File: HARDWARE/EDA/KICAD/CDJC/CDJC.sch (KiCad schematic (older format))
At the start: 68 parts

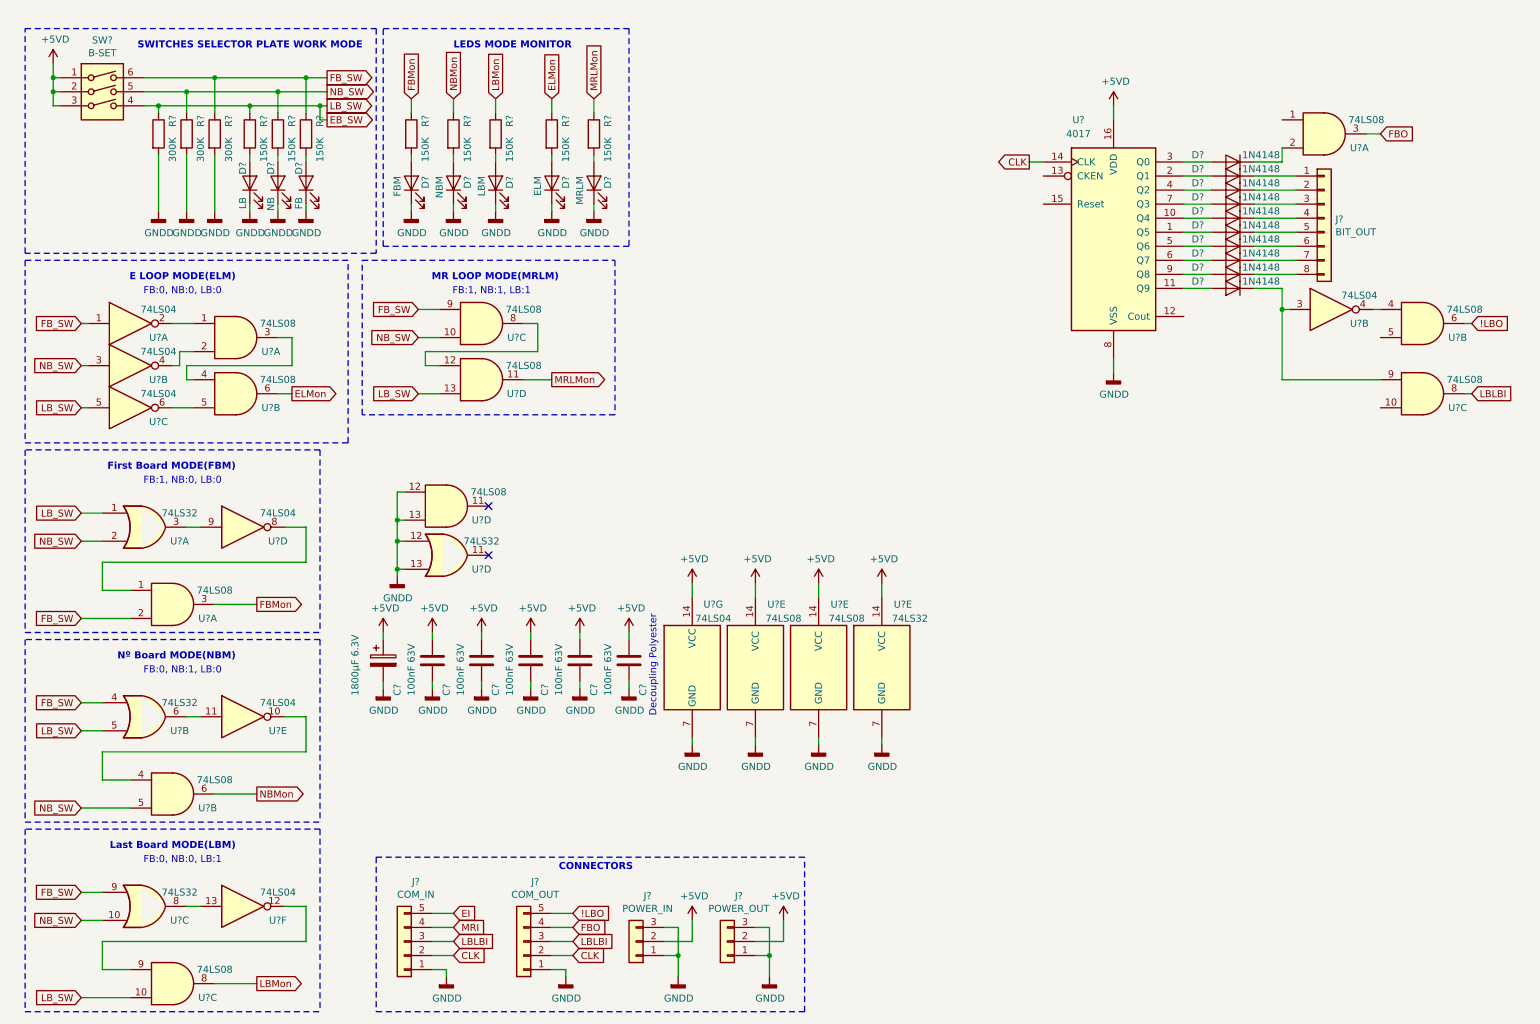
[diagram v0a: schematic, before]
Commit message: finished project
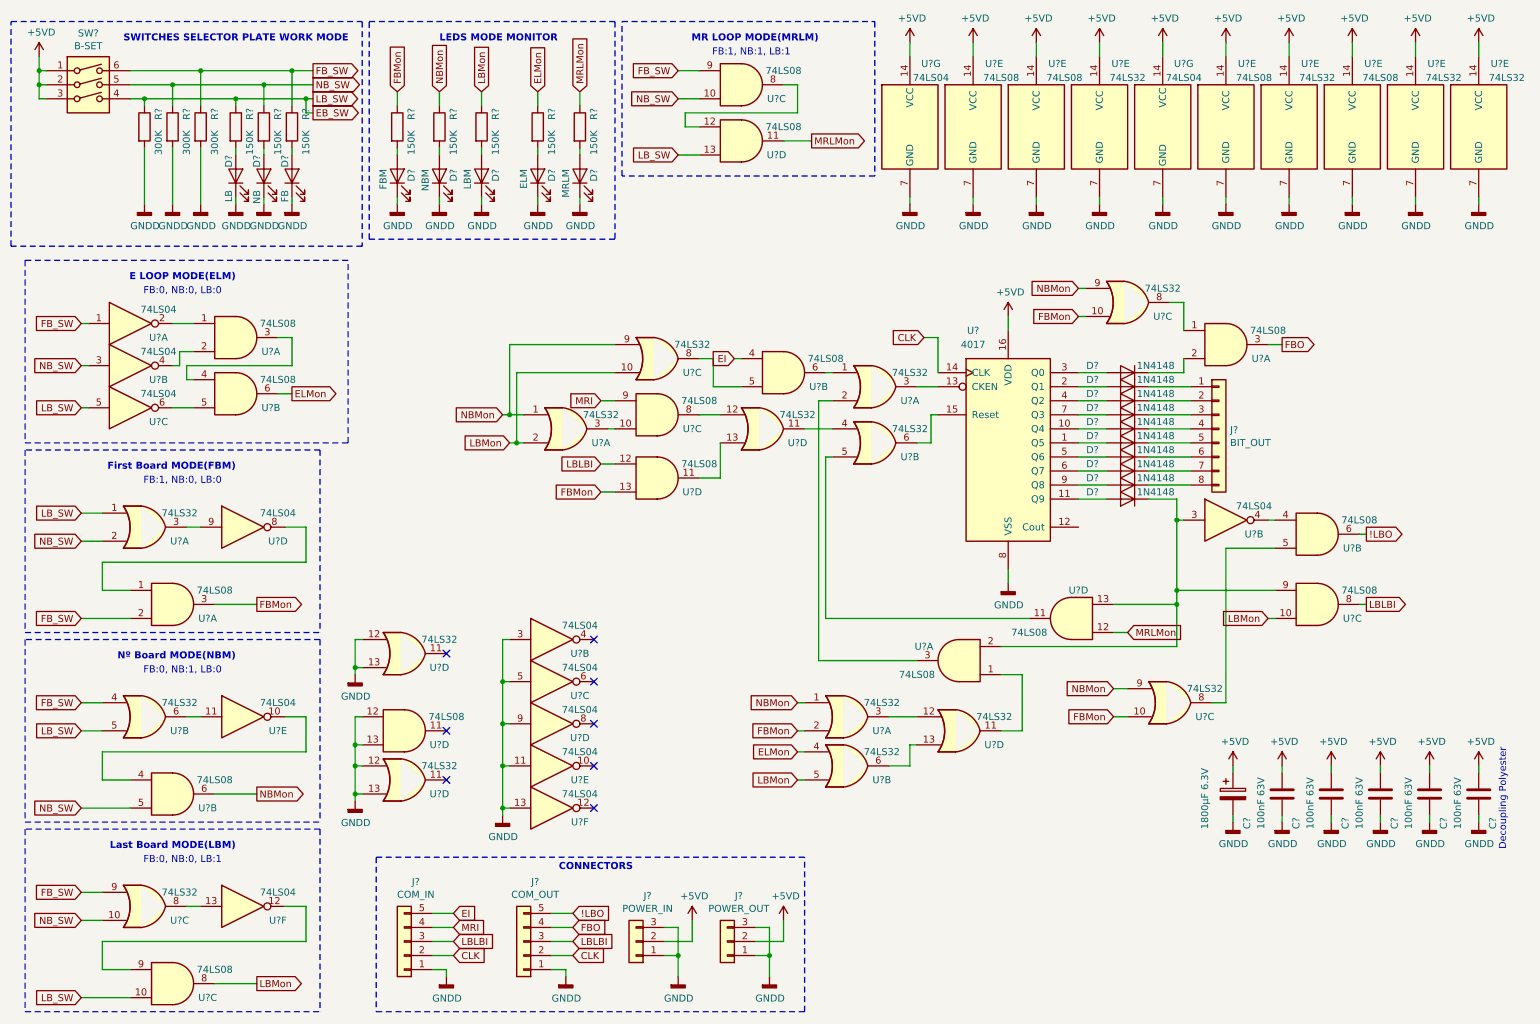
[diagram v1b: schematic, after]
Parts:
- added U? (x14): 74LS32, symbol 74xx:74LS32
- added U? (x7): 74LS08, symbol 74xx:74LS08
- added U? (x6): 74LS04, symbol 74xx:74LS04
- J?: footprint Connector_PinHeader_2.00mm:PinHeader_1x03_P2.00mm_Horizontal -> Connector_PinSocket_2.00mm:PinSocket_1x03_P2.00mm_Horizontal
- J?: footprint Connector_PinHeader_2.00mm:PinHeader_1x05_P2.00mm_Horizontal -> Connector_PinSocket_2.00mm:PinSocket_1x05_P2.00mm_Horizontal
- J?: footprint Connector_PinHeader_2.00mm:PinHeader_1x08_P2.00mm_Horizontal -> Connector_PinSocket_2.00mm:PinSocket_1x08_P2.00mm_Horizontal
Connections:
- net +5VD: now also U?.14 (VCC), U?.14 (VCC), U?.14 (VCC), U?.14 (VCC), U?.14 (VCC), U?.14 (VCC)
- net EI: now also U?.4
- net ELMon: now also U?.4
- net FBMon: now also U?.10, U?.10, U?.13, U?.2
- net GNDD: now also U?.11, U?.12, U?.13, U?.13, U?.3, U?.5, U?.7 (GND), U?.7 (GND), U?.7 (GND), U?.7 (GND), U?.7 (GND), U?.7 (GND), U?.9
- net LBLBI: now also U?.12
- net LBMon: now also U?.10, U?.10, U?.2, U?.5
- net MRI: now also U?.9
- net MRLMon: now also U?.12
- net NBMon: now also U?.1, U?.1, U?.9, U?.9, U?.9
- net at U?.13 (CKEN): now also U?.3
- net at U?.15 (Reset): now also U?.6
- net at D?.1 (K), U?.3, U?.9: now also U?.13, U?.2
- net at U?.5: now also U?.8
- net at U?.1: now also U?.8
- new net: U?.10, U?.3
- new net: U?.1, U?.11
- new net: U?.12, U?.3
- new net: U?.13, U?.6
- new net: U?.11, U?.5
- new net: U?.1, U?.6
- new net: U?.2, U?.3
- new net: U?.11, U?.4
- new net: U?.5, U?.8
- new net: U?.12, U?.8
- new net: U?.11, U?.13
- no-connect marks 2 -> 8
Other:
- moved on the sheet: C?, D?, J?, R?, SW?, U?, U?A, U?B, U?C, U?D, U?E, U?G

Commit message: finished project
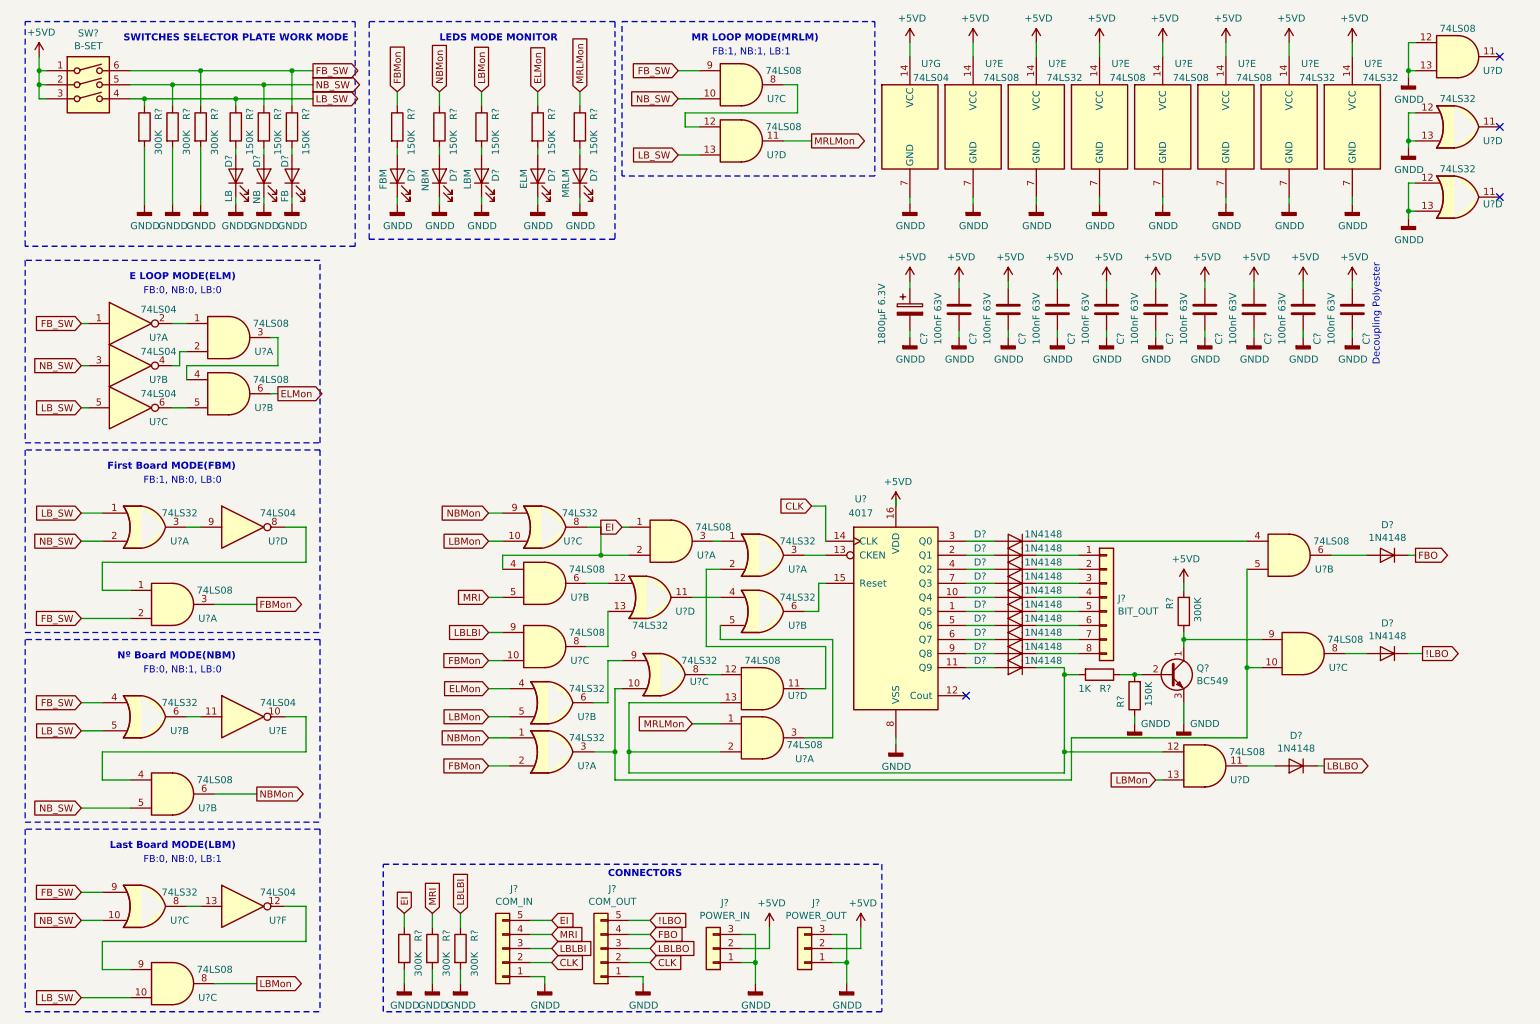
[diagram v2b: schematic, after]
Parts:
- removed C? (x4): 100nF 63V, Capacitor_THT:C_Rect_L7.0mm_W2.5mm_P5.00mm, symbol Device:C
- removed U? (x8): 74LS32, symbol 74xx:74LS32
- removed U? (x4): 74LS08, symbol 74xx:74LS08
- removed U? (x7): 74LS04, symbol 74xx:74LS04
- added C? (x8): 100nF 63V, Capacitor_THT:C_Rect_L7.0mm_W2.5mm_P5.00mm, symbol Device:C
- added D? (x3): 1N4148, Diode_THT:D_DO-35_SOD27_P7.62mm_Horizontal, symbol Diode:1N4148
- added Q?: BC549, Package_TO_SOT_THT:TO-92_Inline, symbol Transistor_BJT:BC549
- added R? (x4): 300K, Resistor_THT:R_Axial_DIN0207_L6.3mm_D2.5mm_P7.62mm_Horizontal, symbol Device:R
- added R?: 1K, Resistor_THT:R_Axial_DIN0207_L6.3mm_D2.5mm_P7.62mm_Horizontal, symbol Device:R
- added R?: 150K, Resistor_THT:R_Axial_DIN0207_L6.3mm_D2.5mm_P7.62mm_Horizontal, symbol Device:R
- added U? (x4): 74LS08, Package_DIP:DIP-14_W7.62mm_LongPads, symbol 74xx:74LS08
- added U? (x4): 74LS32, Package_DIP:DIP-14_W7.62mm_LongPads, symbol 74xx:74LS32
- U? (x34): footprint (none) -> Package_DIP:DIP-14_W7.62mm_LongPads
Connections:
- net !LBO: now also D?.1 (K); no longer U?.6
- net +5VD: now also C?.1, C?.1, C?.1, C?.1, C?.1, C?.1, C?.1, C?.1, R?.2, U?.14 (VCC), U?.14 (VCC), U?.14 (VCC), U?.14 (VCC), U?.14 (VCC)
- net EI: now also U?.1, R?.1; no longer U?.4
- net FBMon: now also U?.10; no longer U?.13
- net FBO: now also D?.1 (K); no longer U?.3
- net GNDD: now also C?.2, C?.2, C?.2, C?.2, C?.2, C?.2, C?.2, C?.2, Q?.3 (E), R?.1, R?.2, R?.2, R?.2, U?.12, U?.12, U?.12, U?.13, U?.13, U?.13, U?.7 (GND), U?.7 (GND), U?.7 (GND), U?.7 (GND), U?.7 (GND)
- net LBLBI: now also U?.9, R?.1; no longer J?.3 (Pin_3), U?.12, U?.8
- net LBMon: now also U?.10, U?.13; no longer U?.10, U?.2
- net MRI: now also U?.5, R?.1; no longer U?.9
- net MRLMon: now also U?.1; no longer U?.12
- net NBMon: now also U?.9; no longer U?.1
- net at U?.3: now also U?.10, U?.10, U?.5; no longer U?.12
- net at U?.6: now also U?.9; no longer U?.13
- net at D?.1 (K): now also U?.4; no longer U?.2
- net at U?.5: now also U?.3; no longer U?.11
- net at U?.1: now also U?.3; no longer U?.6
- net at U?.2: now also U?.11; no longer U?.3
- net at U?.12: now also U?.6; no longer U?.8
- net at U?.13: now also U?.8; no longer U?.11
- net EB_SW renamed LB_SW
- new net: U?.2, U?.4, U?.8
- new net: U?.12, U?.8
- new net: D?.1 (K), R?.2, U?.12, U?.13, U?.2
- new net: D?.2 (A), U?.8
- new net: Q?.1 (C), R?.1, U?.9
- new net: D?.2 (A), U?.6
- new net: D?.2 (A), U?.11
- new net: Q?.2 (B), R?.1, R?.2
- new net LBLBO: D?.1 (K), J?.3 (Pin_3)
- no-connect marks 8 -> 4
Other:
- moved on the sheet: C?, D?, J?, U?, U?A, U?B, U?D, U?E
